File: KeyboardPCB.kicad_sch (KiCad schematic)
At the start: 21 parts, among them J1 AVR-ISP-6, SW68 SW_SKQG, U1 ATmega32U4-A, Y1 Crystal_GND24_Small

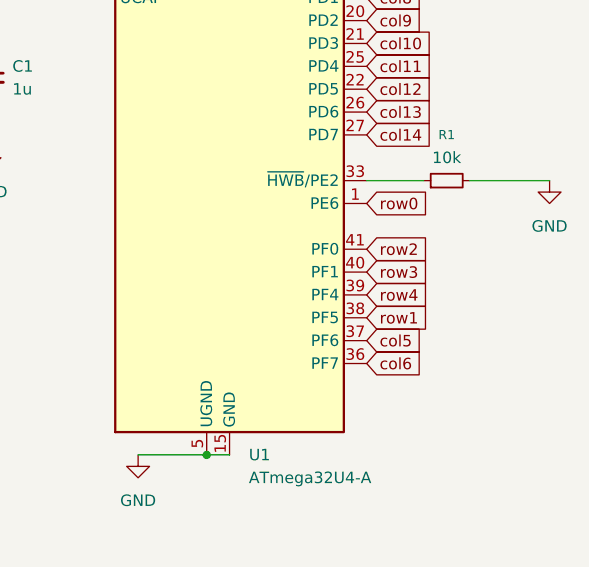
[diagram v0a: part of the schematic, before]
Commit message: Continued routing
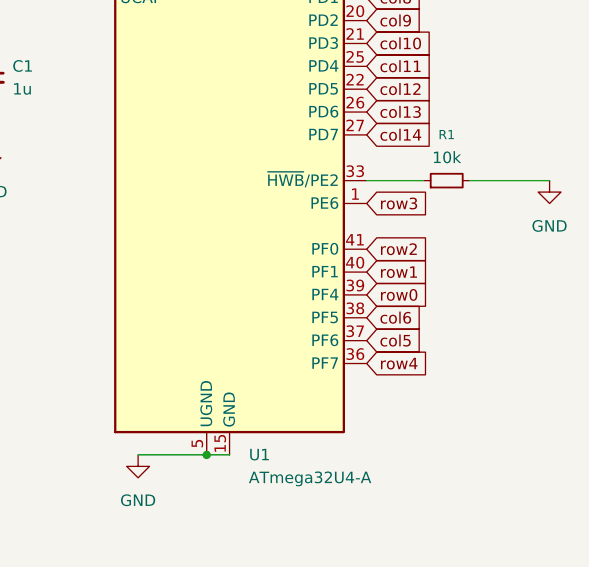
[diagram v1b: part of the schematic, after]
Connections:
- net col6: now also U1.38 (PF5); no longer U1.36 (PF7)
- net row0: now also U1.39 (PF4); no longer U1.1 (PE6)
- net row1: now also U1.40 (PF1); no longer U1.38 (PF5)
- net row3: now also U1.1 (PE6); no longer U1.40 (PF1)
- net row4: now also U1.36 (PF7); no longer U1.39 (PF4)
